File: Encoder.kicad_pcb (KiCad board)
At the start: 2 copper layers, 23.5 x 26 mm, 17 parts, among them J1 Conn_01x05_Pin, SW1 RotaryEncoder_Switch_MP, U1 74LVC3G14

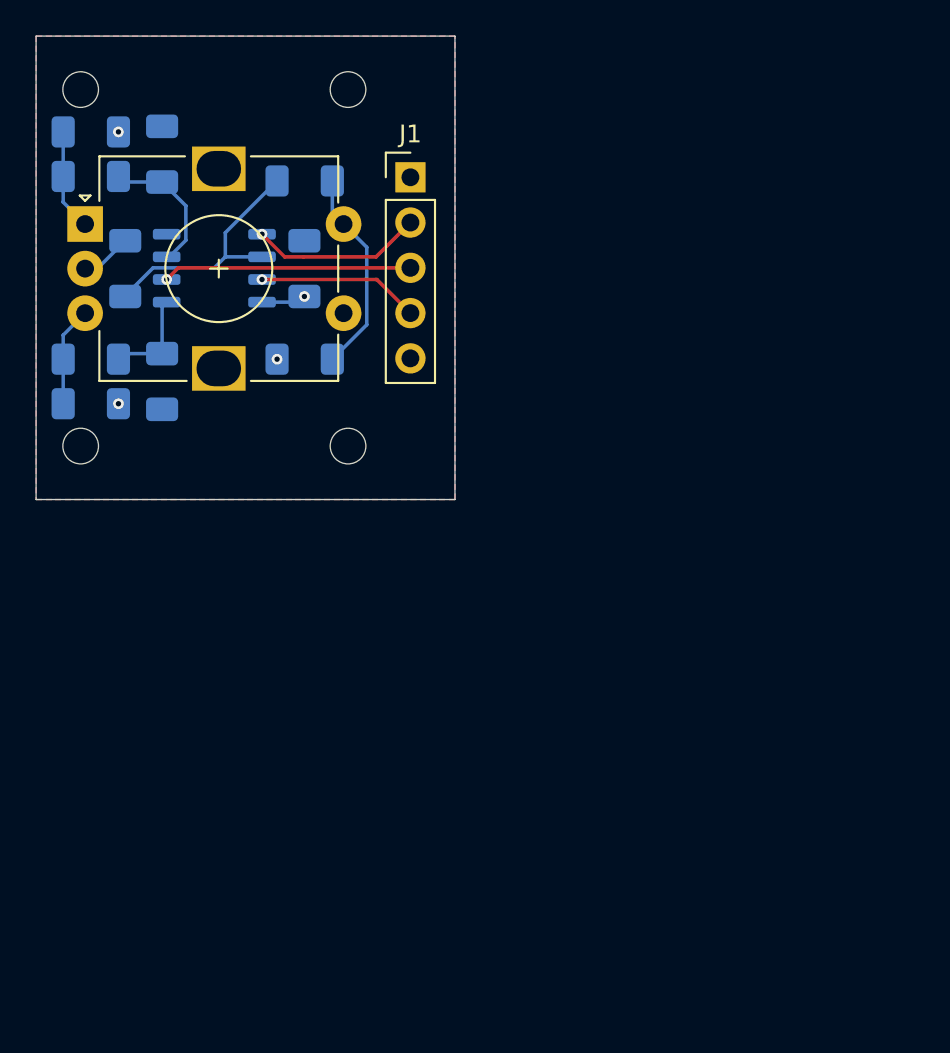
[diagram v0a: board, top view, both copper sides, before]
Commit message: Layout done
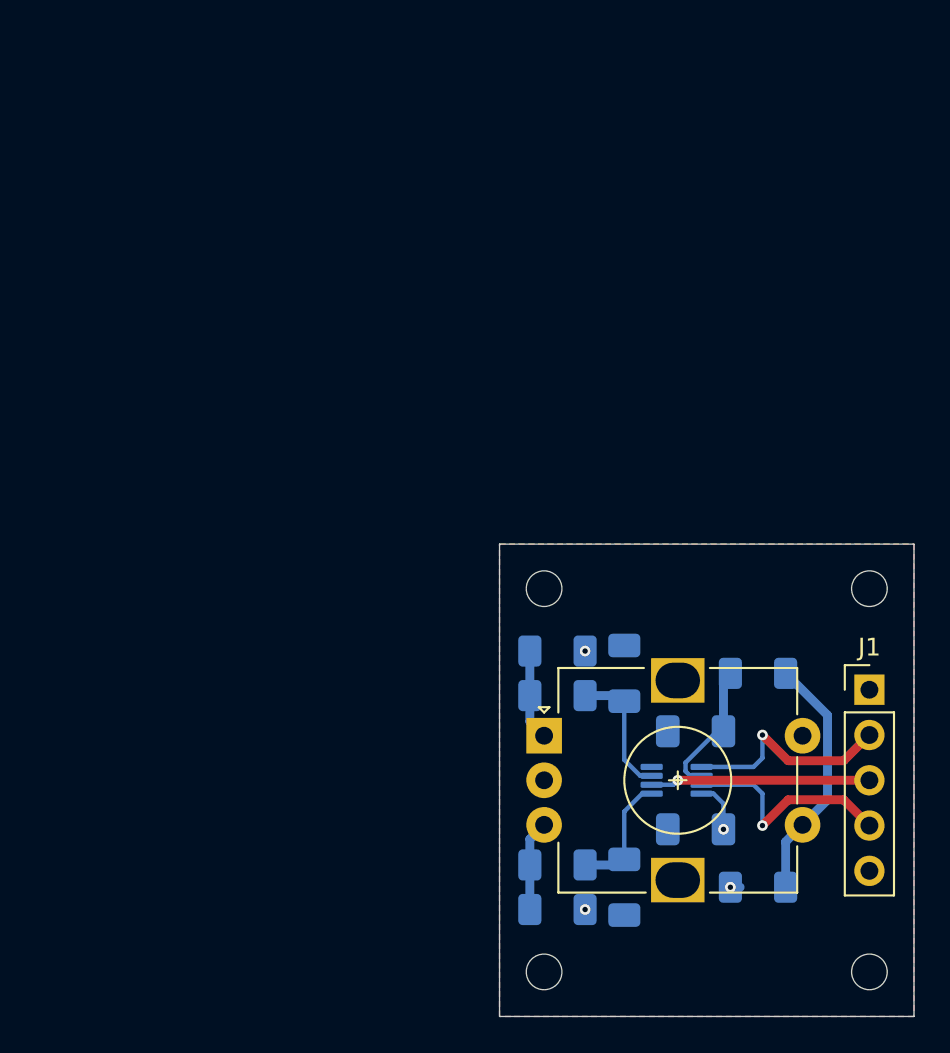
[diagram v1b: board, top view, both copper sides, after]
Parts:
- U1: footprint Package_SO:SSOP-8_3.9x5.05mm_P1.27mm -> Package_SO:VSSOP-8_2.3x2mm_P0.5mm
- moved H3 55.9 mm to (145.0, 122.0)
- moved H2 41.5 mm to (163.2, 122.0)
- moved C1 41.2 mm to (153.5, 108.5), turned to 180 degrees
- moved H1 40.5 mm to (163.2, 100.5)
- moved R3 39.2 mm to (145.8, 106.5)
- moved R4 39.2 mm to (145.8, 104.0)
- moved R1 39.0 mm to (157.0, 117.2)
- moved C2 39.0 mm to (149.5, 105.2)
- moved U1 38.7 mm to (152.4, 111.2)
- moved R5 38.6 mm to (145.8, 116.0)
- moved R6 38.6 mm to (145.8, 118.5)
- moved J1 38.6 mm to (163.2, 106.2)
- moved SW1 38.6 mm to (145.0, 108.8)
- moved C3 38.4 mm to (149.5, 117.2)
- moved C4 38.4 mm to (153.5, 114.0), turned to 180 degrees
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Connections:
- SW1 pad S1: /BTN -> GND
- SW1 pad S2: GND -> /BTN
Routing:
- net Net-(C1-Pad1): track 14.1 -> 7.76 mm
- net /Debounced.B: track 9.11 -> 12.6 mm
- net GND: track 2.90 -> 0.00 mm
- net /Debounced.A: track 9.65 -> 12.1 mm
- net /BTN: track 11.6 -> 13.9 mm
- net /Debounced.BTN: track 13.9 -> 12.3 mm
- net Net-(C3-Pad1): track 5.57 -> 6.97 mm
- net VCC: track 2.51 -> 3.45 mm
- net /A: track 5.68 -> 5.08 mm
- net /B: track 5.59 -> 5.08 mm
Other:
- board size 23.5 x 26 mm -> 23.2 x 26.5 mm
